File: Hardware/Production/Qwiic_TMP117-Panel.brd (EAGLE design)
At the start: 22.9 x 24.1 mm, 43 parts, among them J1 PTH, U2 TMP117

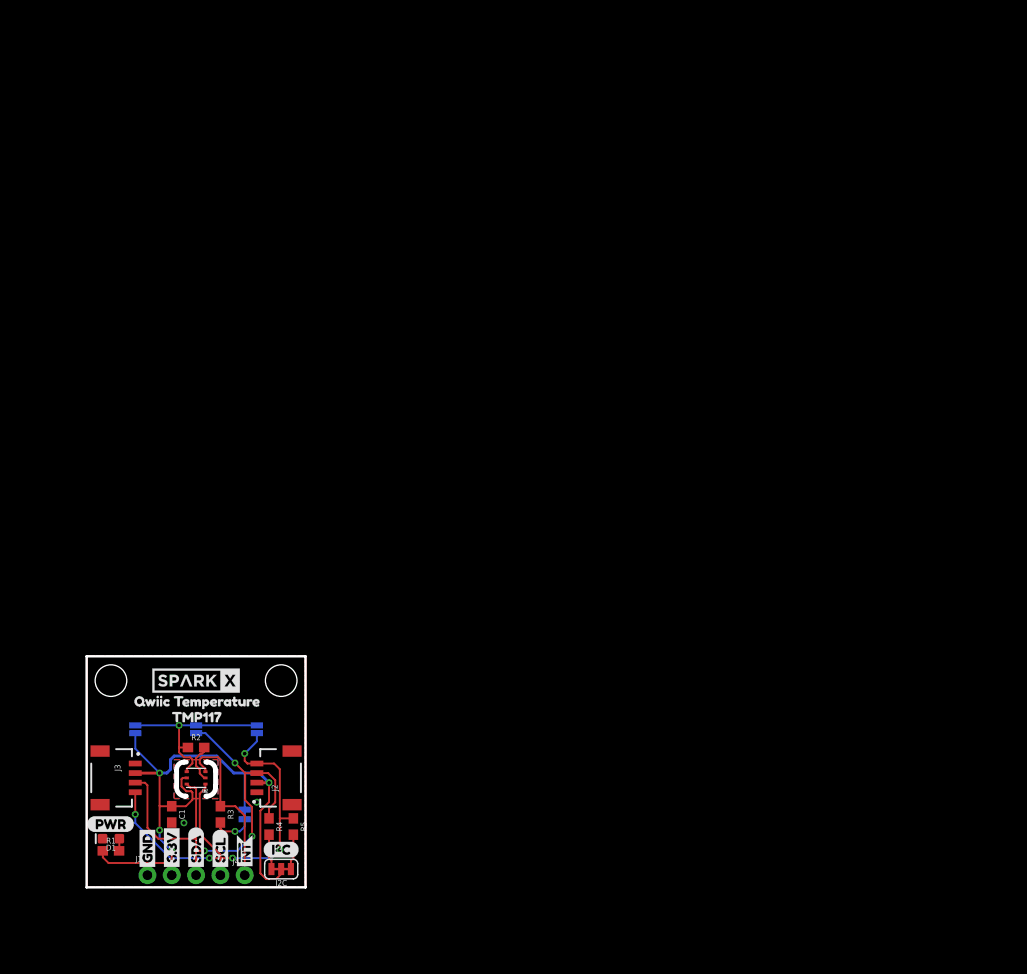
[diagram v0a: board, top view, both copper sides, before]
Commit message: Final Design
Final updated board with the production panelized board and Gerber files
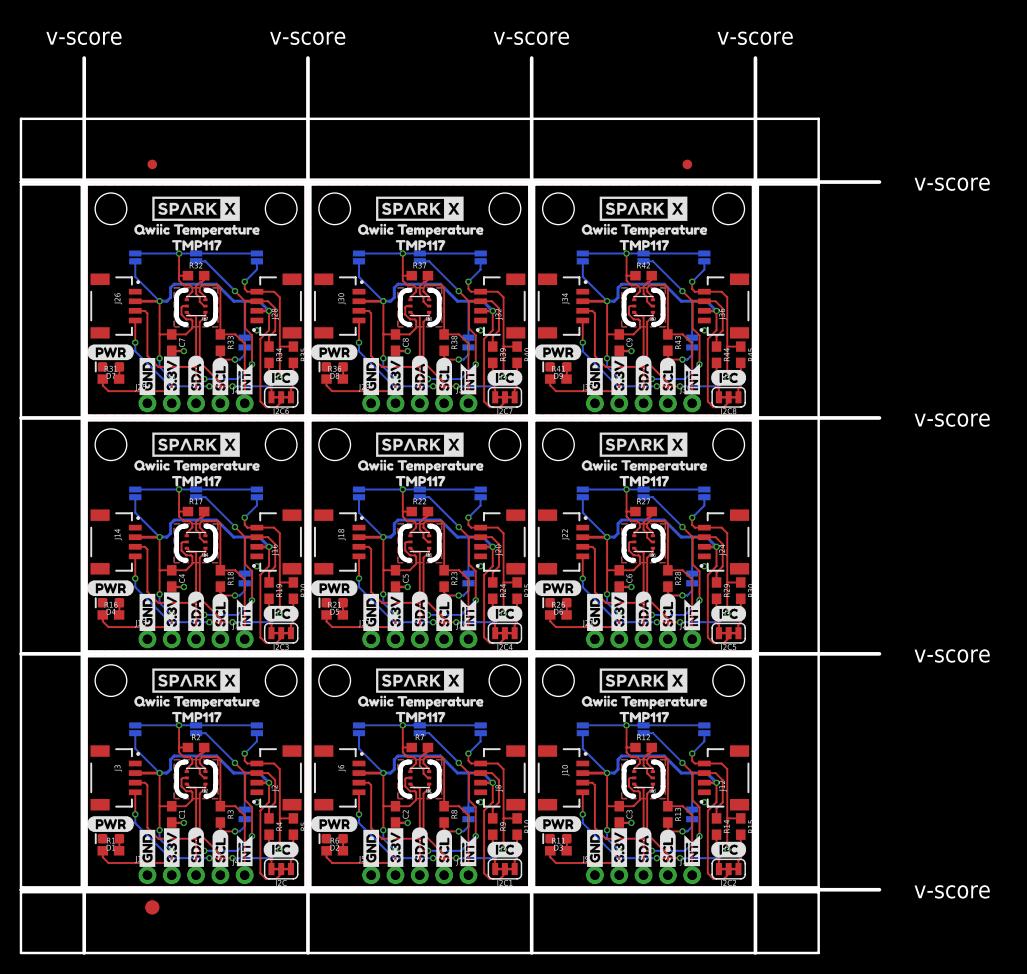
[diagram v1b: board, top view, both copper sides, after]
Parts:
- removed FRAME1: FRAME-LETTER, SparkFun-Aesthetics:CREATIVE_COMMONS
- added C2, C3, C4, C5, C6, C7, C8, C9: 0.1uF, SparkFun-Capacitors:0603
- added D2, D3, D4, D5, D6, D7, D8, D9: RED, SparkFun-LED:LED-0603
- added E$1, E$2: (no value), SparkFun-Aesthetics:FIDUCIAL-1X2
- added E$3: (no value), SparkFun-Retired:FIDUCIAL-1.5X3
- added I2C1, I2C2, I2C3, I2C4, I2C5, I2C6, I2C7, I2C8: (no value), SparkFun-Jumpers:SMT-JUMPER_3_2-NC_TRACE_SILK
- added J10, J12, J14, J16, J18, J20, J22, J24, J26, J28, J30, J32, J34, J36, J6, J8: (no value), SparkFun-Connectors:JST04_1MM_RA
- added J11, J15, J19, J23, J27, J31, J35, J7: (no value), SparkFun-Connectors:1X01_NO_SILK
- added J13, J17, J21, J25, J29, J33, J5, J9: PTH, SparkX:1X04_NO_SILK
- added JP11, JP16, JP17, JP22, JP23, JP28, JP29, JP34, JP35, JP40, JP41, JP46, JP47, JP52, JP53, JP7: STAND-OFF, SparkFun:STAND-OFF
- added JP12, JP18, JP24, JP30, JP36, JP42, JP48, JP54: INT, SparkFun-Passives:PAD-JUMPER-2-NC_BY_TRACE_YES_SILK
- added JP13, JP14, JP15, JP19, JP20, JP21, JP25, JP26, JP27, JP31, JP32, JP33, JP37, JP38, JP39, JP4, JP43, JP44, JP45, JP49, JP5, JP50, JP51, JP6: (no value), SparkFun-Jumpers:SMT-JUMPER_2_NO_SILK
- added LOGO2, LOGO3, LOGO4, LOGO5, LOGO6, LOGO7, LOGO8, LOGO9: OSHW-LOGOMINI, SparkFun-Aesthetics:OSHW-LOGO-MINI
- added R10, R14, R15, R19, R20, R24, R25, R29, R30, R34, R35, R39, R40, R44, R45, R9: 2.2k, SparkFun-Resistors:0603
- added R11, R16, R21, R26, R31, R36, R41, R6: 1k, SparkFun-Resistors:0603
- added R12, R13, R17, R18, R22, R23, R27, R28, R32, R33, R37, R38, R42, R43, R7, R8: 10k, SparkFun-Resistors:0603
- added U$100, U$121, U$122, U$143, U$144, U$165, U$166, U$187, U$188, U$33, U$34, U$55, U$56, U$77, U$78, U$99: (no value), Labels:3.3V
- added U$101, U$102, U$123, U$124, U$145, U$146, U$167, U$168, U$189, U$190, U$35, U$36, U$57, U$58, U$79, U$80: (no value), Labels:GND-04
- added U$103, U$117, U$125, U$139, U$147, U$161, U$169, U$183, U$191, U$29, U$37, U$51, U$59, U$73, U$81, U$95: (no value), Labels:SCL-[)
- added U$104, U$105, U$126, U$127, U$148, U$149, U$170, U$171, U$192, U$193, U$38, U$39, U$60, U$61, U$82, U$83: (no value), Labels:SDA-[)
- added U$106, U$128, U$150, U$172, U$194, U$40, U$62, U$84: (no value), buzzard_labels (15):0X4B1
- added U$107, U$129, U$151, U$173, U$195, U$41, U$63, U$85: (no value), buzzard_labels (15):0X4A0
- added U$108, U$130, U$152, U$174, U$196, U$42, U$64, U$86: (no value), buzzard_labels (15):0X493
- added U$109, U$131, U$153, U$175, U$197, U$43, U$65, U$87: (no value), buzzard_labels (15):ADR_#_0X484
- added U$110, U$132, U$154, U$176, U$198, U$44, U$66, U$88: (no value), SparkFun-Aesthetics:QWIIC_5.5MM
- added U$111, U$133, U$155, U$16, U$177, U$45, U$67, U$89: (no value), buzzard_labels:TMP1171
- added U$112, U$134, U$156, U$178, U$24, U$46, U$68, U$90: (no value), buzzard_labels (2):QWIIC_TEMPERATURE2
- added U$113, U$114, U$135, U$136, U$157, U$158, U$179, U$180, U$25, U$26, U$47, U$48, U$69, U$70, U$91, U$92: (no value), SparkX:SPARKX-MEDIUM
- added U$115, U$118, U$137, U$140, U$159, U$162, U$181, U$184, U$27, U$30, U$49, U$52, U$71, U$74, U$93, U$96: (no value), Labels:INT#-[<-04
- added U$116, U$138, U$160, U$182, U$28, U$50, U$72, U$94: (no value), Labels:INT-()-04
- added U$119, U$141, U$163, U$185, U$31, U$53, U$75, U$97: (no value), Labels:PWR-()-04
- added U$120, U$142, U$164, U$186, U$32, U$54, U$76, U$98: (no value), Labels:I_SUPER2_C-()-04
- added U1, U3, U4, U5, U6, U7, U8, U9: TMP117, TMP117:TMP117
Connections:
- new net !INT1: J7.1, R8.1, U1.3
- new net !INT2: J11.1, R13.1, U3.3
- new net !INT3: J15.1, R18.1, U4.3
- new net !INT4: J19.1, R23.1, U5.3
- new net !INT5: J23.1, R28.1, U6.3
- new net !INT6: J27.1, R33.1, U7.3
- new net !INT7: J31.1, R38.1, U8.3
- new net !INT8: J35.1, R43.1, U9.3
- new net 3.3V1: C2.1, I2C1.2, J5.2, J6.2, J8.2, JP12.2, JP6.2, R6.1, U1.5
- new net 3.3V2: C3.1, I2C2.2, J10.2, J12.2, J9.2, JP15.2, JP18.2, R11.1, U3.5
- new net 3.3V3: C4.1, I2C3.2, J13.2, J14.2, J16.2, JP21.2, JP24.2, R16.1, U4.5
- new net 3.3V4: C5.1, I2C4.2, J17.2, J18.2, J20.2, JP27.2, JP30.2, R21.1, U5.5
- new net 3.3V5: C6.1, I2C5.2, J21.2, J22.2, J24.2, JP33.2, JP36.2, R26.1, U6.5
- new net 3.3V6: C7.1, I2C6.2, J25.2, J26.2, J28.2, JP39.2, JP42.2, R31.1, U7.5
- new net 3.3V7: C8.1, I2C7.2, J29.2, J30.2, J32.2, JP45.2, JP48.2, R36.1, U8.5
- new net 3.3V8: C9.1, I2C8.2, J33.2, J34.2, J36.2, JP51.2, JP54.2, R41.1, U9.5
- new net ADD1: JP4.1, JP5.1, JP6.1, R7.1, U1.4
- new net ADD2: JP13.1, JP14.1, JP15.1, R12.1, U3.4
- new net ADD3: JP19.1, JP20.1, JP21.1, R17.1, U4.4
- new net ADD4: JP25.1, JP26.1, JP27.1, R22.1, U5.4
- new net ADD5: JP31.1, JP32.1, JP33.1, R27.1, U6.4
- new net ADD6: JP37.1, JP38.1, JP39.1, R32.1, U7.4
- new net ADD7: JP43.1, JP44.1, JP45.1, R37.1, U8.4
- new net ADD8: JP49.1, JP50.1, JP51.1, R42.1, U9.4
- new net GND1: C2.2, D2.C, J5.1, J6.1, J8.1, R7.2, U1.2
- new net GND2: C3.2, D3.C, J10.1, J12.1, J9.1, R12.2, U3.2
- new net GND3: C4.2, D4.C, J13.1, J14.1, J16.1, R17.2, U4.2
- new net GND4: C5.2, D5.C, J17.1, J18.1, J20.1, R22.2, U5.2
- new net GND5: C6.2, D6.C, J21.1, J22.1, J24.1, R27.2, U6.2
- new net GND6: C7.2, D7.C, J25.1, J26.1, J28.1, R32.2, U7.2
- new net GND7: C8.2, D8.C, J29.1, J30.1, J32.1, R37.2, U8.2
- new net GND8: C9.2, D9.C, J33.1, J34.1, J36.1, R42.2, U9.2
- new net N$10: JP12.1, R8.2
- new net N$13: D3.A, R11.2
- new net N$14: I2C2.1, R15.2
- new net N$15: I2C2.3, R14.2
- new net N$16: JP18.1, R13.2
- new net N$19: D4.A, R16.2
- new net N$20: I2C3.1, R20.2
- new net N$21: I2C3.3, R19.2
- new net N$22: JP24.1, R18.2
- new net N$25: D5.A, R21.2
- new net N$26: I2C4.1, R25.2
- new net N$27: I2C4.3, R24.2
- new net N$28: JP30.1, R23.2
- new net N$31: D6.A, R26.2
- new net N$32: I2C5.1, R30.2
- new net N$33: I2C5.3, R29.2
- new net N$34: JP36.1, R28.2
- new net N$37: D7.A, R31.2
- new net N$38: I2C6.1, R35.2
- new net N$39: I2C6.3, R34.2
- new net N$40: JP42.1, R33.2
- new net N$43: D8.A, R36.2
- new net N$44: I2C7.1, R40.2
- new net N$45: I2C7.3, R39.2
- new net N$46: JP48.1, R38.2
- new net N$49: D9.A, R41.2
- new net N$50: I2C8.1, R45.2
- new net N$51: I2C8.3, R44.2
- new net N$52: JP54.1, R43.2
- new net N$7: D2.A, R6.2
- new net N$8: I2C1.1, R10.2
- new net N$9: I2C1.3, R9.2
- new net SCL1: J5.4, J6.4, J8.4, JP4.2, R10.1, U1.1
- new net SCL2: J10.4, J12.4, J9.4, JP13.2, R15.1, U3.1
- new net SCL3: J13.4, J14.4, J16.4, JP19.2, R20.1, U4.1
- new net SCL4: J17.4, J18.4, J20.4, JP25.2, R25.1, U5.1
- new net SCL5: J21.4, J22.4, J24.4, JP31.2, R30.1, U6.1
- new net SCL6: J25.4, J26.4, J28.4, JP37.2, R35.1, U7.1
- new net SCL7: J29.4, J30.4, J32.4, JP43.2, R40.1, U8.1
- new net SCL8: J33.4, J34.4, J36.4, JP49.2, R45.1, U9.1
- new net SDA1: J5.3, J6.3, J8.3, JP5.2, R9.1, U1.6
- new net SDA2: J10.3, J12.3, J9.3, JP14.2, R14.1, U3.6
- new net SDA3: J13.3, J14.3, J16.3, JP20.2, R19.1, U4.6
- new net SDA4: J17.3, J18.3, J20.3, JP26.2, R24.1, U5.6
- new net SDA5: J21.3, J22.3, J24.3, JP32.2, R29.1, U6.6
- new net SDA6: J25.3, J26.3, J28.3, JP38.2, R34.1, U7.6
- new net SDA7: J29.3, J30.3, J32.3, JP44.2, R39.1, U8.6
- new net SDA8: J33.3, J34.3, J36.3, JP50.2, R44.1, U9.6
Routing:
- net 3.3V4: track 0.00 -> 66.3 mm, vias 0 -> 4
- net 3.3V3: track 0.00 -> 66.3 mm, vias 0 -> 4
- net 3.3V1: track 0.00 -> 66.3 mm, vias 0 -> 4
- net 3.3V7: track 0.00 -> 66.3 mm, vias 0 -> 4
- net 3.3V5: track 0.00 -> 66.3 mm, vias 0 -> 4
- net 3.3V2: track 0.00 -> 66.3 mm, vias 0 -> 4
- net 3.3V6: track 0.00 -> 66.3 mm, vias 0 -> 4
- net 3.3V8: track 0.00 -> 66.3 mm, vias 0 -> 4
- net SDA8: track 0.00 -> 49.5 mm, vias 0 -> 3
- net SDA7: track 0.00 -> 49.5 mm, vias 0 -> 3
- net SDA6: track 0.00 -> 49.5 mm, vias 0 -> 3
- net SDA3: track 0.00 -> 49.5 mm, vias 0 -> 3
- net SDA2: track 0.00 -> 49.5 mm, vias 0 -> 3
- net SDA5: track 0.00 -> 49.5 mm, vias 0 -> 3
- net SDA4: track 0.00 -> 49.5 mm, vias 0 -> 3
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- added copper zone on layer 1, net GND1
- added copper zone on layer 16, net GND1
- added copper zone on layer 1, net GND2
- added copper zone on layer 16, net GND2
- added copper zone on layer 1, net GND3
- added copper zone on layer 16, net GND3
- added copper zone on layer 1, net GND4
- added copper zone on layer 16, net GND4
- added copper zone on layer 1, net GND5
- added copper zone on layer 16, net GND5
- added copper zone on layer 1, net GND6
- added copper zone on layer 16, net GND6
- added copper zone on layer 1, net GND7
- added copper zone on layer 16, net GND7
- added copper zone on layer 1, net GND8
- added copper zone on layer 16, net GND8
- added copper zone on layer 1, net N$11
- added copper zone on layer 16, net N$12
- added copper zone on layer 1, net N$17
- added copper zone on layer 16, net N$18
- added copper zone on layer 1, net N$23
- added copper zone on layer 16, net N$24
- added copper zone on layer 1, net N$29
- added copper zone on layer 16, net N$30
- added copper zone on layer 1, net N$35
- added copper zone on layer 16, net N$36
- added copper zone on layer 1, net N$41
- added copper zone on layer 16, net N$42
- added copper zone on layer 1, net N$47
- added copper zone on layer 16, net N$48
- added copper zone on layer 1, net N$53
- added copper zone on layer 16, net N$54
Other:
- board size 22.9 x 24.1 mm -> 89.7 x 93.5 mm
- board text added: "v-score"
- board text removed: "Madison Chodikov"
